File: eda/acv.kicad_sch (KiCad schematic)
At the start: 6 parts, among them J1 OBD2, J2 CAN TRANS, U1 ESP32-C6-DevKitC-1

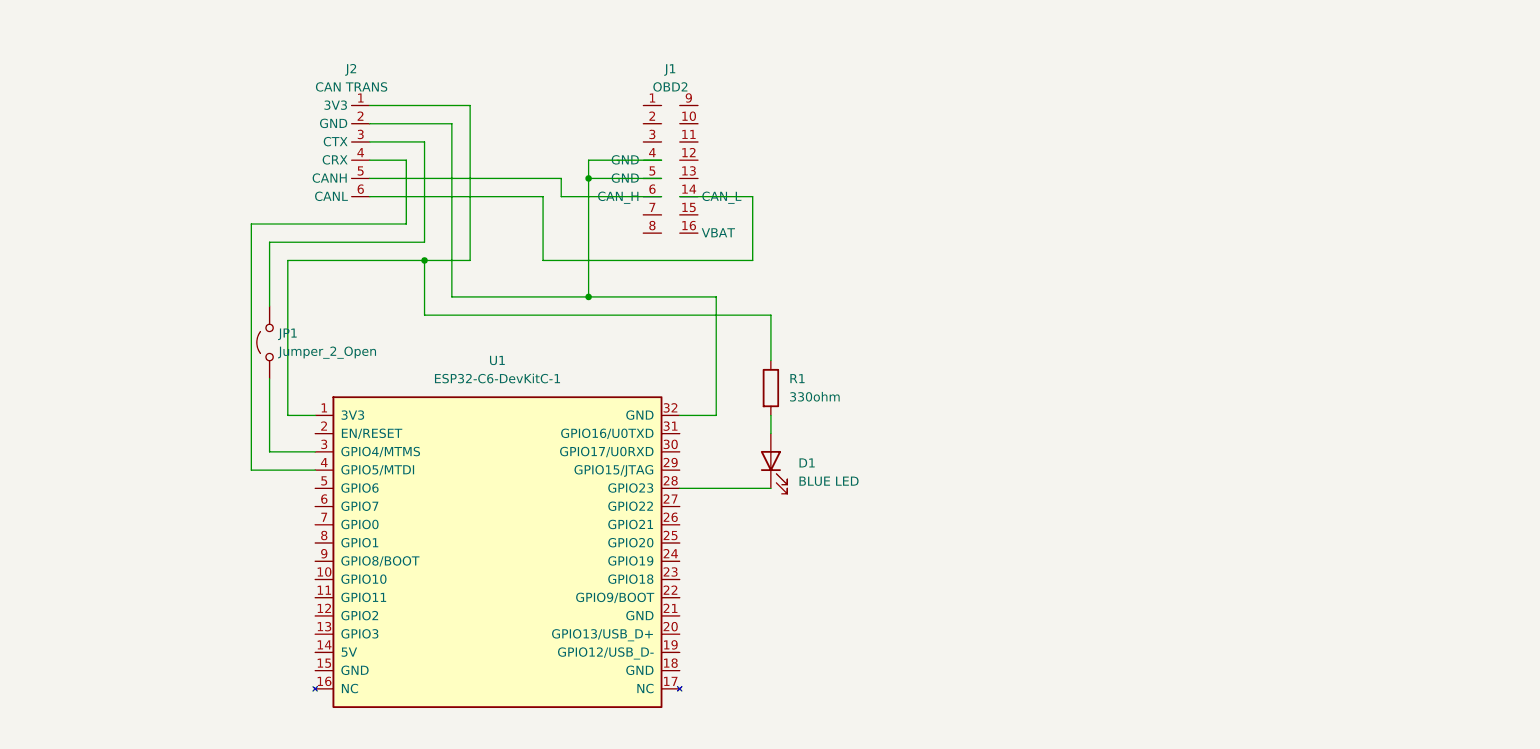
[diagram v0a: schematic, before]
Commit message: Update EDA
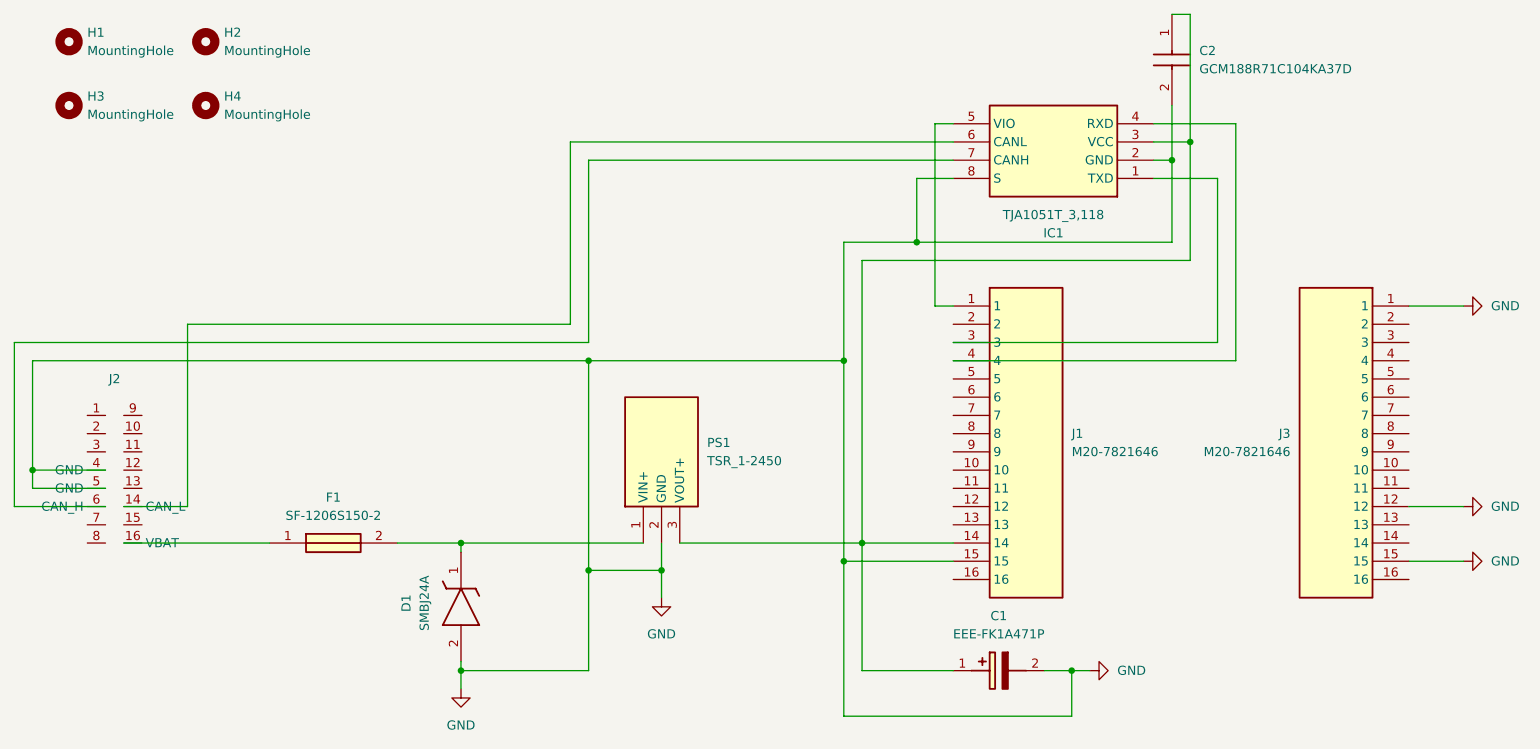
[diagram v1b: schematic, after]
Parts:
- removed D1: BLUE LED, symbol Device:LED
- removed J1: OBD2, symbol acv:OBD2_J1962_MALE_90
- removed J2: CAN TRANS, symbol acv:SN65HVD230
- removed JP1: Jumper_2_Open, symbol Jumper:Jumper_2_Open
- removed R1: 330ohm, symbol Device:R
- removed U1: ESP32-C6-DevKitC-1, PCM_Espressif:ESP32-C6-DevKitC-1, symbol Espressif:ESP32-C6-DevKitC-1
- added C1: EEE-FK1A471P, acv:EEHZT1E331UP, symbol acv:EEE-FK1A471P
- added C2: GCM188R71C104KA37D, CAPC1608X90N, symbol acv:GCM188R71C104KA37D
- added D1: SMBJ24A, acv:DIOM5436X261N, symbol acv:SMBJ24A
- added F1: SF-1206S150-2, acv:FUSC3116X70N, symbol acv:SF-1206S150-2
- added H1, H2, H3, H4: MountingHole, MountingHole:MountingHole_2.2mm_M2, symbol Mechanical:MountingHole
- added IC1: TJA1051T_3,118, acv:SOIC127P600X175-8N, symbol acv:TJA1051T_3,118
- added J1, J3: M20-7821646, acv:RHDR16W70P0X254_1X16_4104X250X850P, symbol acv:M20-7821646
- added J2: ~, acv:OBD2_J1962_MALE_90, symbol acv:OBD2_J1962_MALE_90
- added PS1: TSR_1-2450, TSR-1-24120, symbol acv:TSR_1-2450
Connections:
- new net: IC1.5 (VIO), J1.1
- new net: C1.1 (+), C2.1, IC1.3 (VCC), J1.14, PS1.3 (VOUT+)
- new net: IC1.1 (TXD), J1.3
- new net: IC1.4 (RXD), J1.4
- new net: F1.1, J2.16 (VBAT)
- new net: D1.1 (K), F1.2, PS1.1 (VIN+)
- new net: IC1.6 (CANL), J2.14 (CAN_L)
- new net: IC1.7 (CANH), J2.6 (CAN_H)
- new net GND: C1.2 (-), C2.2, D1.2 (A), IC1.2 (GND), IC1.8 (S), J1.15, J2.4 (GND), J2.5 (GND), J3.1, J3.12, J3.15, PS1.2 (GND)
